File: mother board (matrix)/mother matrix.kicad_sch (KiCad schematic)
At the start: 0 parts

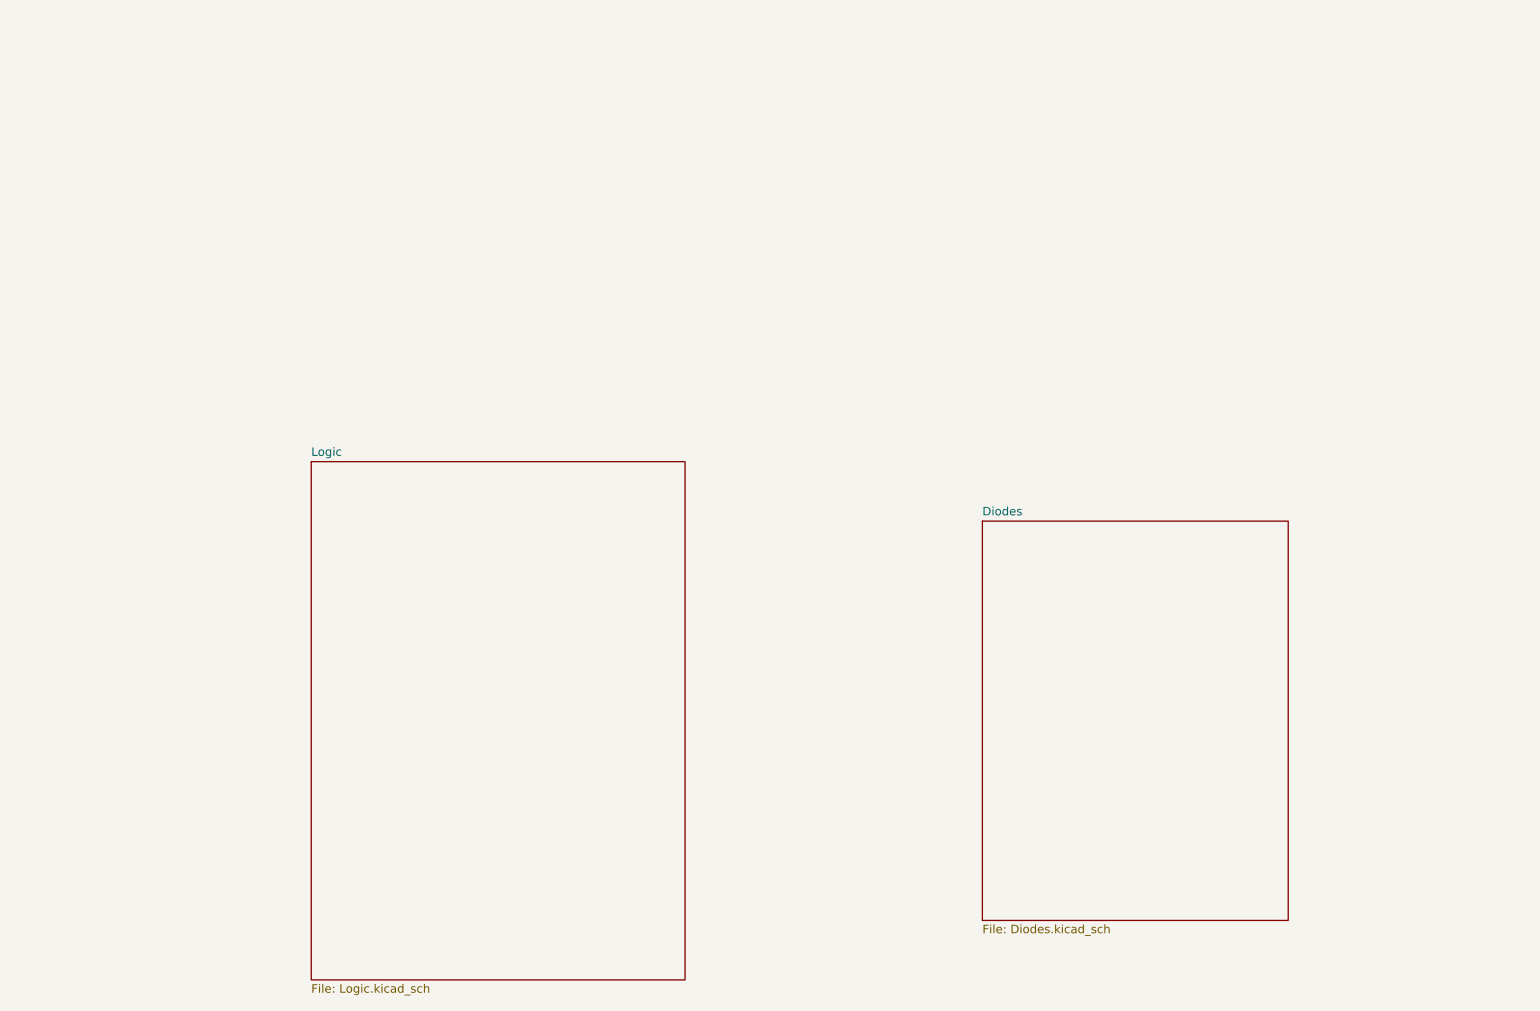
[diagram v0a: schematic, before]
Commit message: matrix done
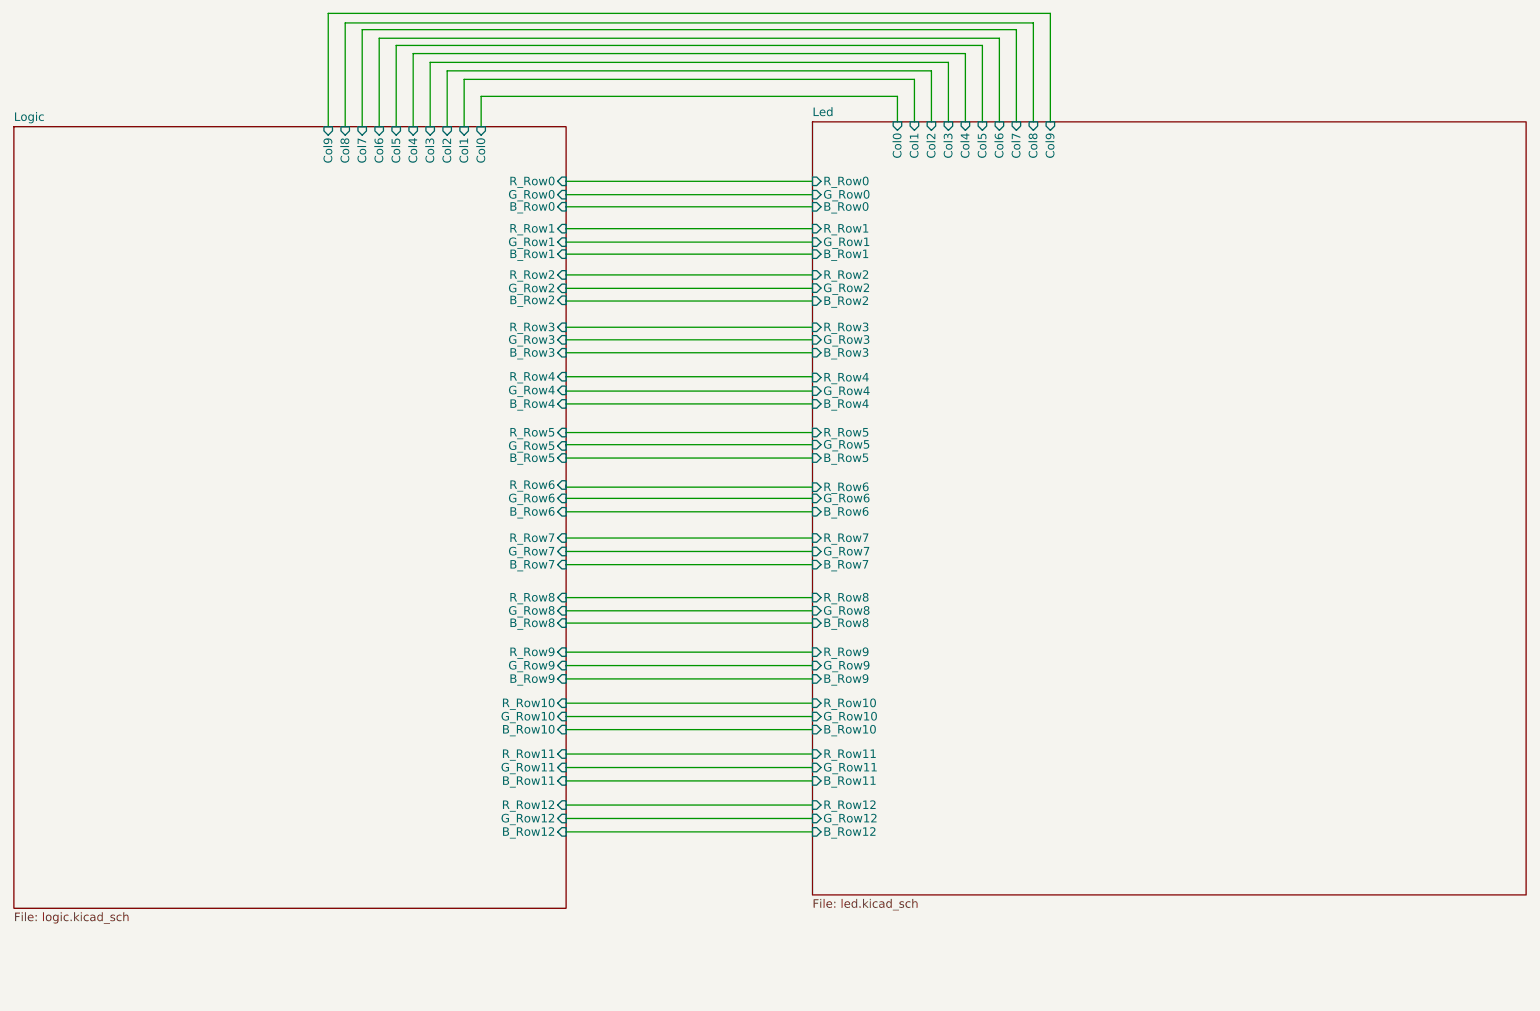
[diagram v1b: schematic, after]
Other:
- removed sheet Diodes
- added sheet Led (led.kicad_sch)
- sheet Logic: file Logic.kicad_sch -> logic.kicad_sch
- sheet Logic ports: added B_Row0, B_Row1, B_Row10, B_Row11, B_Row12, B_Row2, B_Row3, B_Row4, B_Row5, B_Row6, B_Row7, B_Row8, B_Row9, Col0, Col1, Col2, Col3, Col4, Col5, Col6, Col7, Col8, Col9, G_Row0, G_Row1, G_Row10, G_Row11, G_Row12, G_Row2, G_Row3, G_Row4, G_Row5, G_Row6, G_Row7, G_Row8, G_Row9, R_Row0, R_Row1, R_Row10, R_Row11, R_Row12, R_Row2, R_Row3, R_Row4, R_Row5, R_Row6, R_Row7, R_Row8, R_Row9; removed none
